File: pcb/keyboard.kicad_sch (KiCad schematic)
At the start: 132 parts, among them SW1 SW_Push_45deg, SW10 SW_Push_45deg, SW11 SW_Push_45deg, SW12 SW_Push_45deg, SW13 SW_Push_45deg, SW14 SW_Push_45deg, SW15 SW_Push_45deg, SW16 SW_Push_45deg, SW17 SW_Push_45deg, SW18 SW_Push_45deg, SW19 SW_Push_45deg, SW2 SW_Push_45deg, SW20 SW_Push_45deg, SW21 SW_Push_45deg, SW22 SW_Push_45deg, SW23 SW_Push_45deg, SW24 SW_Push_45deg, SW25 SW_Push_45deg, SW26 SW_Push_45deg, SW27 SW_Push_45deg, SW28 SW_Push_45deg, SW29 SW_Push_45deg, SW3 SW_Push_45deg, SW30 SW_Push_45deg, SW31 SW_Push_45deg, SW32 SW_Push_45deg, SW33 SW_Push_45deg, SW34 SW_Push_45deg, SW35 SW_Push_45deg, SW36 SW_Push_45deg, SW37 SW_Push_45deg, SW38 SW_Push_45deg, SW39 SW_Push_45deg, SW4 SW_Push_45deg, SW40 SW_Push_45deg, SW41 SW_Push_45deg, SW42 SW_Push_45deg, SW43 SW_Push_45deg, SW44 SW_Push_45deg, SW45 SW_Push_45deg, SW46 SW_Push_45deg, SW47 SW_Push_45deg, SW48 SW_Push_45deg, SW49 SW_Push_45deg, SW5 SW_Push_45deg, SW50 SW_Push_45deg, SW51 SW_Push_45deg, SW52 SW_Push_45deg, SW53 SW_Push_45deg, SW54 SW_Push_45deg, SW55 SW_Push_45deg, SW56 SW_Push_45deg, SW57 SW_Push_45deg, SW58 SW_Push_45deg, SW59 SW_Push_45deg, SW6 SW_Push_45deg, SW60 SW_Push_45deg, SW61 SW_Push_45deg, SW62 SW_Push_45deg, SW63 SW_Push_45deg, SW64 SW_Push_45deg, SW65 SW_Push_45deg, SW7 SW_Push_45deg, SW77 RotaryEncoder_Switch, SW8 SW_Push_45deg, SW9 SW_Push_45deg

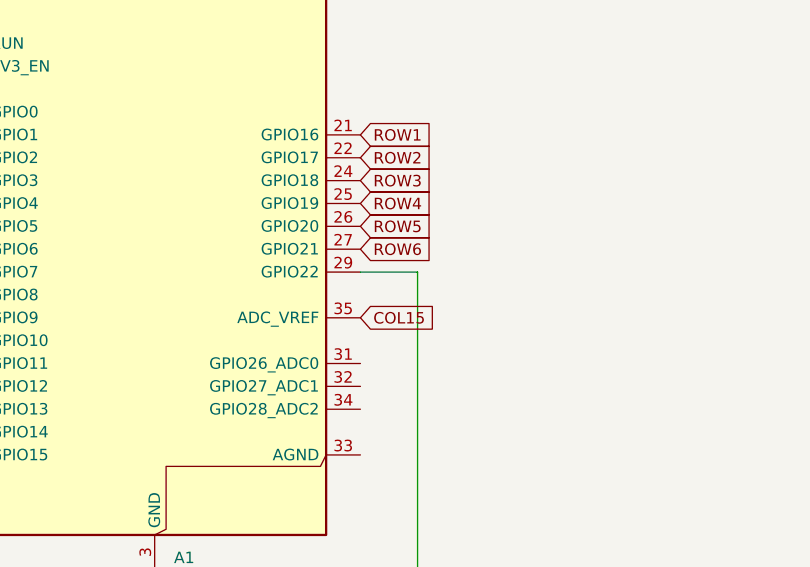
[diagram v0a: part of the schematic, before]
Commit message: updated pcb files
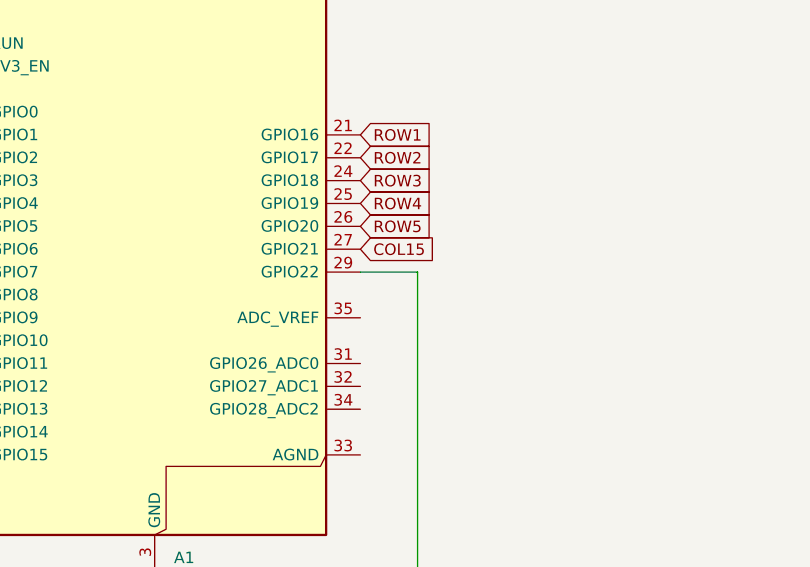
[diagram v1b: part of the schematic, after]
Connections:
- net ROW6 is gone; now on net COL15: A1.27 (GPIO21)
- net COL15: no longer A1.35 (ADC_VREF)
